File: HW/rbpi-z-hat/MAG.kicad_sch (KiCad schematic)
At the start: 0 parts

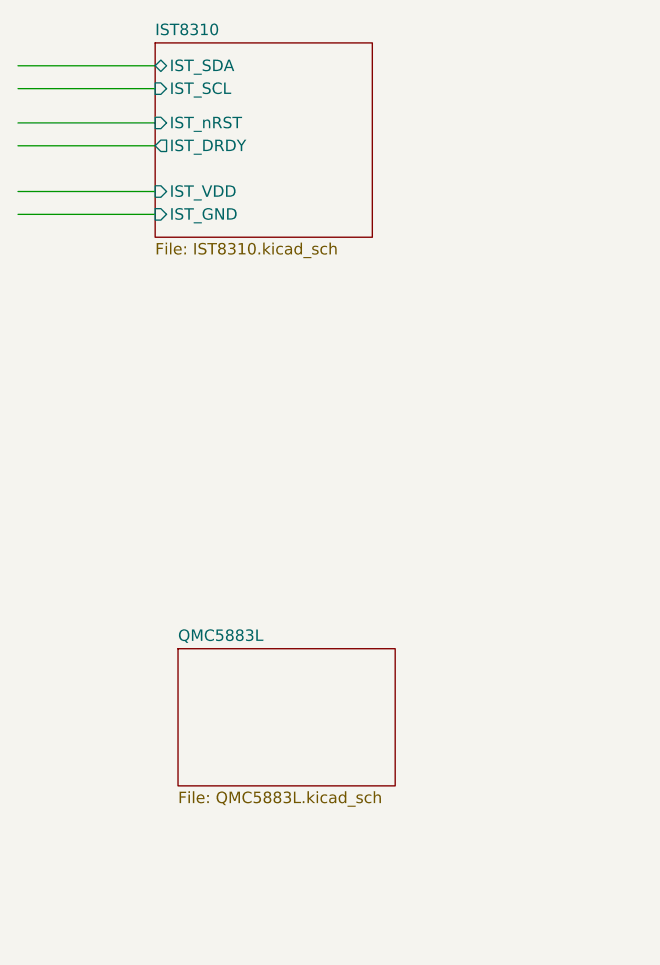
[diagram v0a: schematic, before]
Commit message: Apdated Sch and PCB
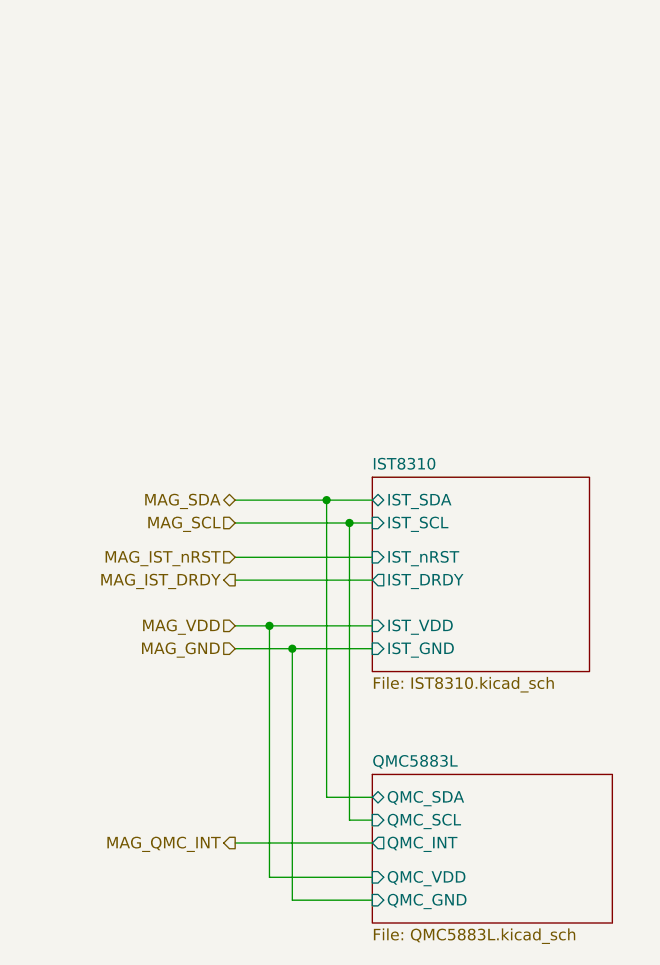
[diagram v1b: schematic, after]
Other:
- sheet QMC5883L ports: added QMC_GND, QMC_INT, QMC_SCL, QMC_SDA, QMC_VDD; removed none
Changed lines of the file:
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@@
     (comment 2 "Denis Tsekh")
   )
-  (wire (pts (xy 67.31 93.98) (xy 82.55 93.98))
+  (junction (at 95.25 139.7) (diameter 0) (color 0 0 0 0)
+  )
+  (junction (at 104.14 128.27) (diameter 0) (color 0 0 0 0)
+  )
+  (junction (at 97.79 142.24) (diameter 0) (color 0 0 0 0)
+  )
+  (junction (at 101.6 125.73) (diameter 0) (color 0 0 0 0)
+  )
+  (wire (pts (xy 91.44 142.24) (xy 97.79 142.24))
     (stroke (width 0) (type default))
   )
-  (wire (pts (xy 67.31 77.47) (xy 82.55 77.47))
+  (wire (pts (xy 91.44 125.73) (xy 101.6 125.73))
     (stroke (width 0) (type default))
   )
-  (wire (pts (xy 67.31 83.82) (xy 82.55 83.82))
+  (wire (pts (xy 104.14 128.27) (xy 106.68 128.27))
     (stroke (width 0) (type default))
   )
-  (wire (pts (xy 67.31 80.01) (xy 82.55 80.01))
+  (wire (pts (xy 91.44 132.08) (xy 106.68 132.08))
     (stroke (width 0) (type default))
   )
-  (wire (pts (xy 67.31 86.36) (xy 82.55 86.36))
+  (wire (pts (xy 104.14 128.27) (xy 104.14 161.29))
     (stroke (width 0) (type default))
   )
-  (wire (pts (xy 67.31 91.44) (xy 82.55 91.44))
+  (wire (pts (xy 91.44 128.27) (xy 104.14 128.27))
     (stroke (width 0) (type default))
   )
-  (sheet (at 85.09 142.24) (size 24.13 15.24) (fields_autoplaced)
+  (wire (pts (xy 104.14 161.29) (xy 106.68 161.29))
+    (stroke (width 0) (type default))
+  )
+  (wire (pts (xy 95.25 139.7) (xy 95.25 167.64))
+    (stroke (width 0) (type default))
+  )
+  (wire (pts (xy 97.79 170.18) (xy 106.68 170.18))
+    (stroke (width 0) (type default))
+  )
+  (wire (pts (xy 101.6 158.75) (xy 106.68 158.75))
+    (stroke (width 0) (type default))
+  )
+  (wire (pts (xy 95.25 139.7) (xy 106.68 139.7))
+    (stroke (width 0) (type default))
+  )
+  (wire (pts (xy 91.44 134.62) (xy 106.68 134.62))
+    (stroke (width 0) (type default))
+  )
+  (wire (pts (xy 91.44 163.83) (xy 106.68 163.83))
+    (stroke (width 0) (type default))
+  )
+  (wire (pts (xy 97.79 142.24) (xy 106.68 142.24))
+    (stroke (width 0) (type default))
+  )
+  (wire (pts (xy 95.25 167.64) (xy 106.68 167.64))
+    (stroke (width 0) (type default))
+  )
+  (wire (pts (xy 91.44 139.7) (xy 95.25 139.7))
+    (stroke (width 0) (type default))
+  )
+  (wire (pts (xy 101.6 125.73) (xy 101.6 158.75))
+    (stroke (width 0) (type default))
+  )
+  (wire (pts (xy 97.79 142.24) (xy 97.79 170.18))
+    (stroke (width 0) (type default))
+  )
+  (wire (pts (xy 101.6 125.73) (xy 106.68 125.73))
+    (stroke (width 0) (type default))
+  )
+  (hierarchical_label "MAG_SDA" (shape bidirectional) (at 91.44 125.73 180) (fields_autoplaced)
+    (effects (font (size 1.27 1.27)) (justify right))
+  )
+  (hierarchical_label "MAG_SCL" (shape input) (at 91.44 128.27 180) (fields_autoplaced)
+    (effects (font (size 1.27 1.27)) (justify right))
+  )
+  (hierarchical_label "MAG_GND" (shape input) (at 91.44 142.24 180) (fields_autoplaced)
+    (effects (font (size 1.27 1.27)) (justify right))
+  )
+  (hierarchical_label "MAG_IST_nRST" (shape input) (at 91.44 132.08 180) (fields_autoplaced)
+    (effects (font (size 1.27 1.27)) (justify right))
+  )
+  (hierarchical_label "MAG_VDD" (shape input) (at 91.44 139.7 180) (fields_autoplaced)
+    (effects (font (size 1.27 1.27)) (justify right))
+  )
+  (hierarchical_label "MAG_QMC_INT" (shape output) (at 91.44 163.83 180) (fields_autoplaced)
+    (effects (font (size 1.27 1.27)) (justify right))
+  )
+  (hierarchical_label "MAG_IST_DRDY" (shape output) (at 91.44 134.62 180) (fields_autoplaced)
+    (effects (font (size 1.27 1.27)) (justify right))
+  )
+  (sheet (at 106.68 156.21) (size 26.67 16.51) (fields_autoplaced)
     (stroke (width 0.1524) (type solid))
     (fill (color 0 0 0 0.0000))
-    (property "Sheetname" "QMC5883L" (at 85.09 141.5284 0)
+    (property "Sheetname" "QMC5883L" (at 106.68 155.4984 0)
       (effects (font (size 1.27 1.27)) (justify left bottom))
     )
-    (property "Sheetfile" "QMC5883L.kicad_sch" (at 85.09 158.0646 0)
+    (property "Sheetfile" "QMC5883L.kicad_sch" (at 106.68 173.3046 0)
       (effects (font (size 1.27 1.27)) (justify left top))
+    )
+    (pin "QMC_VDD" input (at 106.68 167.64 180)
+      (effects (font (size 1.27 1.27)) (justify left))
+    )
+    (pin "QMC_SCL" input (at 106.68 161.29 180)
+      (effects (font (size 1.27 1.27)) (justify left))
+    )
+    (pin "QMC_SDA" bidirectional (at 106.68 158.75 180)
+      (effects (font (size 1.27 1.27)) (justify left))
+    )
+    (pin "QMC_GND" input (at 106.68 170.18 180)
+      (effects (font (size 1.27 1.27)) (justify left))
+    )
+    (pin "QMC_INT" output (at 106.68 163.83 180)
+      (effects (font (size 1.27 1.27)) (justify left))
     )
     (instances
@@
     )
   )
-  (sheet (at 82.55 74.93) (size 24.13 21.59) (fields_autoplaced)
+  (sheet (at 106.68 123.19) (size 24.13 21.59) (fields_autoplaced)
     (stroke (width 0.1524) (type solid))
     (fill (color 0 0 0 0.0000))
-    (property "Sheetname" "IST8310" (at 82.55 74.2184 0)
+    (property "Sheetname" "IST8310" (at 106.68 122.4784 0)
       (effects (font (size 1.27 1.27)) (justify left bottom))
     )
-    (property "Sheetfile" "IST8310.kicad_sch" (at 82.55 97.1046 0)
+    (property "Sheetfile" "IST8310.kicad_sch" (at 106.68 145.3646 0)
       (effects (font (size 1.27 1.27)) (justify left top))
     )
-    (pin "IST_GND" input (at 82.55 93.98 180)
+    (pin "IST_GND" input (at 106.68 142.24 180)
       (effects (font (size 1.27 1.27)) (justify left))
     )
-    (pin "IST_VDD" input (at 82.55 91.44 180)
+    (pin "IST_VDD" input (at 106.68 139.7 180)
       (effects (font (size 1.27 1.27)) (justify left))
     )
-    (pin "IST_SDA" bidirectional (at 82.55 77.47 180)
+    (pin "IST_SDA" bidirectional (at 106.68 125.73 180)
       (effects (font (size 1.27 1.27)) (justify left))
     )
-    (pin "IST_SCL" input (at 82.55 80.01 180)
+    (pin "IST_SCL" input (at 106.68 128.27 180)
       (effects (font (size 1.27 1.27)) (justify left))
     )
-    (pin "IST_nRST" input (at 82.55 83.82 180)
+    (pin "IST_nRST" input (at 106.68 132.08 180)
       (effects (font (size 1.27 1.27)) (justify left))
     )
-    (pin "IST_DRDY" output (at 82.55 86.36 180)
+    (pin "IST_DRDY" output (at 106.68 134.62 180)
       (effects (font (size 1.27 1.27)) (justify left))
     )
